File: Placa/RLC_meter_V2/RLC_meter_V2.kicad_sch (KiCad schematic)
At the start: 22 parts, among them J1 Batt1, J2 Batt2, J3 HC05, J4 Load_terminal, U1 LPC845, U2 X9Cxxx, U3 MC33202, U4 AMS1117-3.3

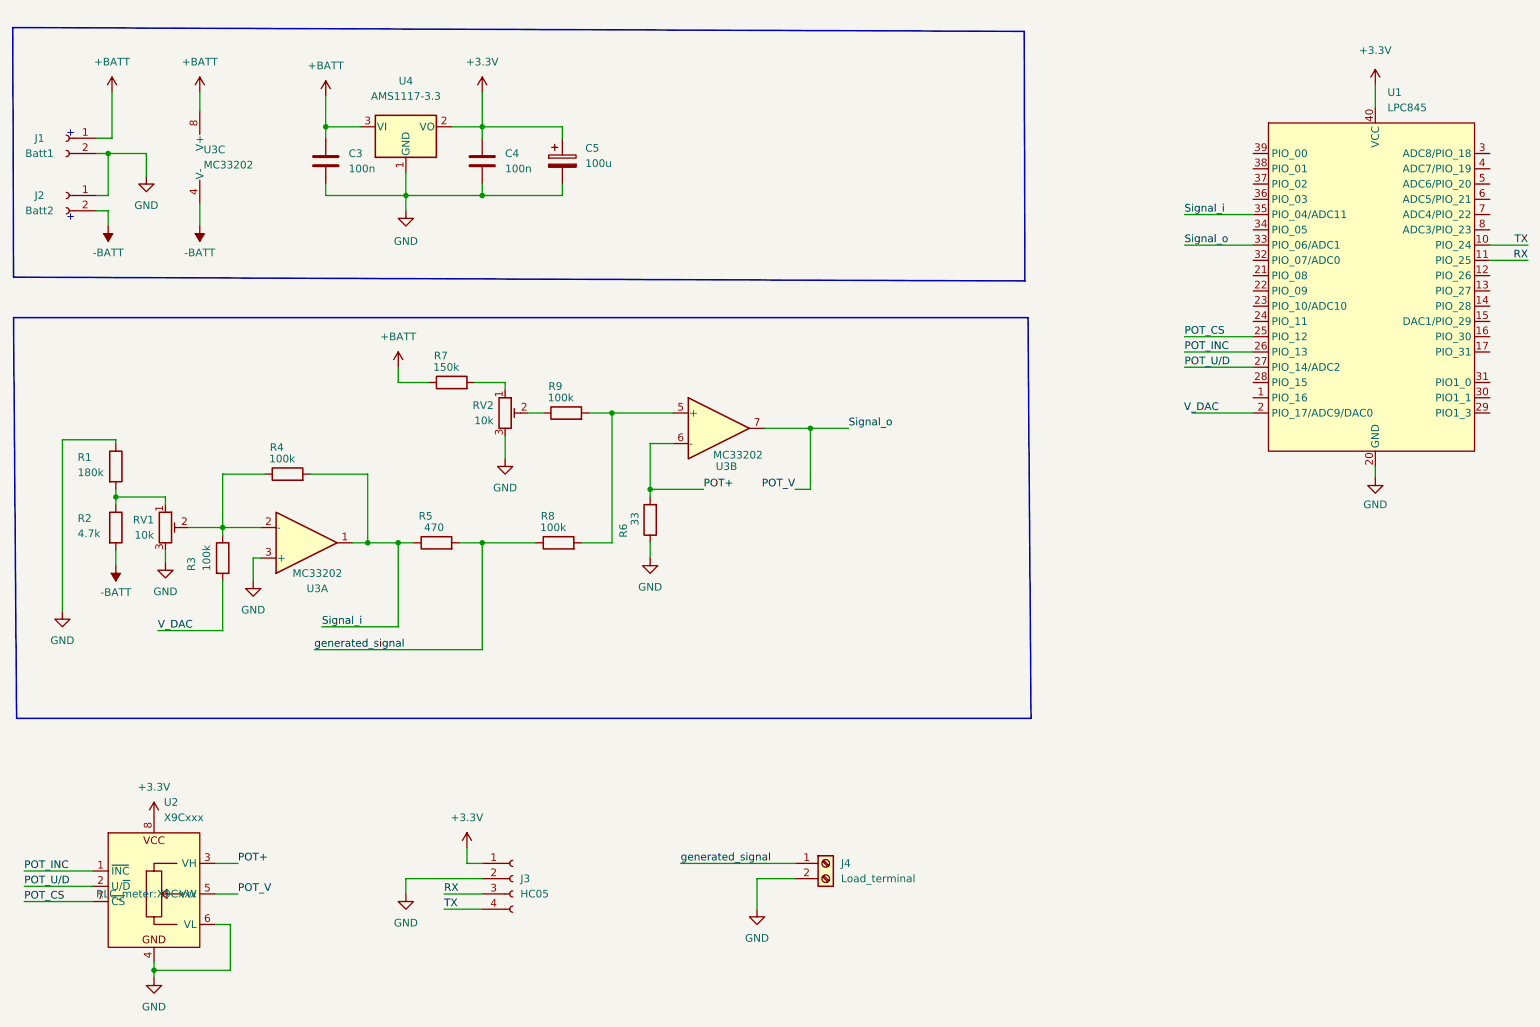
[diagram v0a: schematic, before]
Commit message: last commit
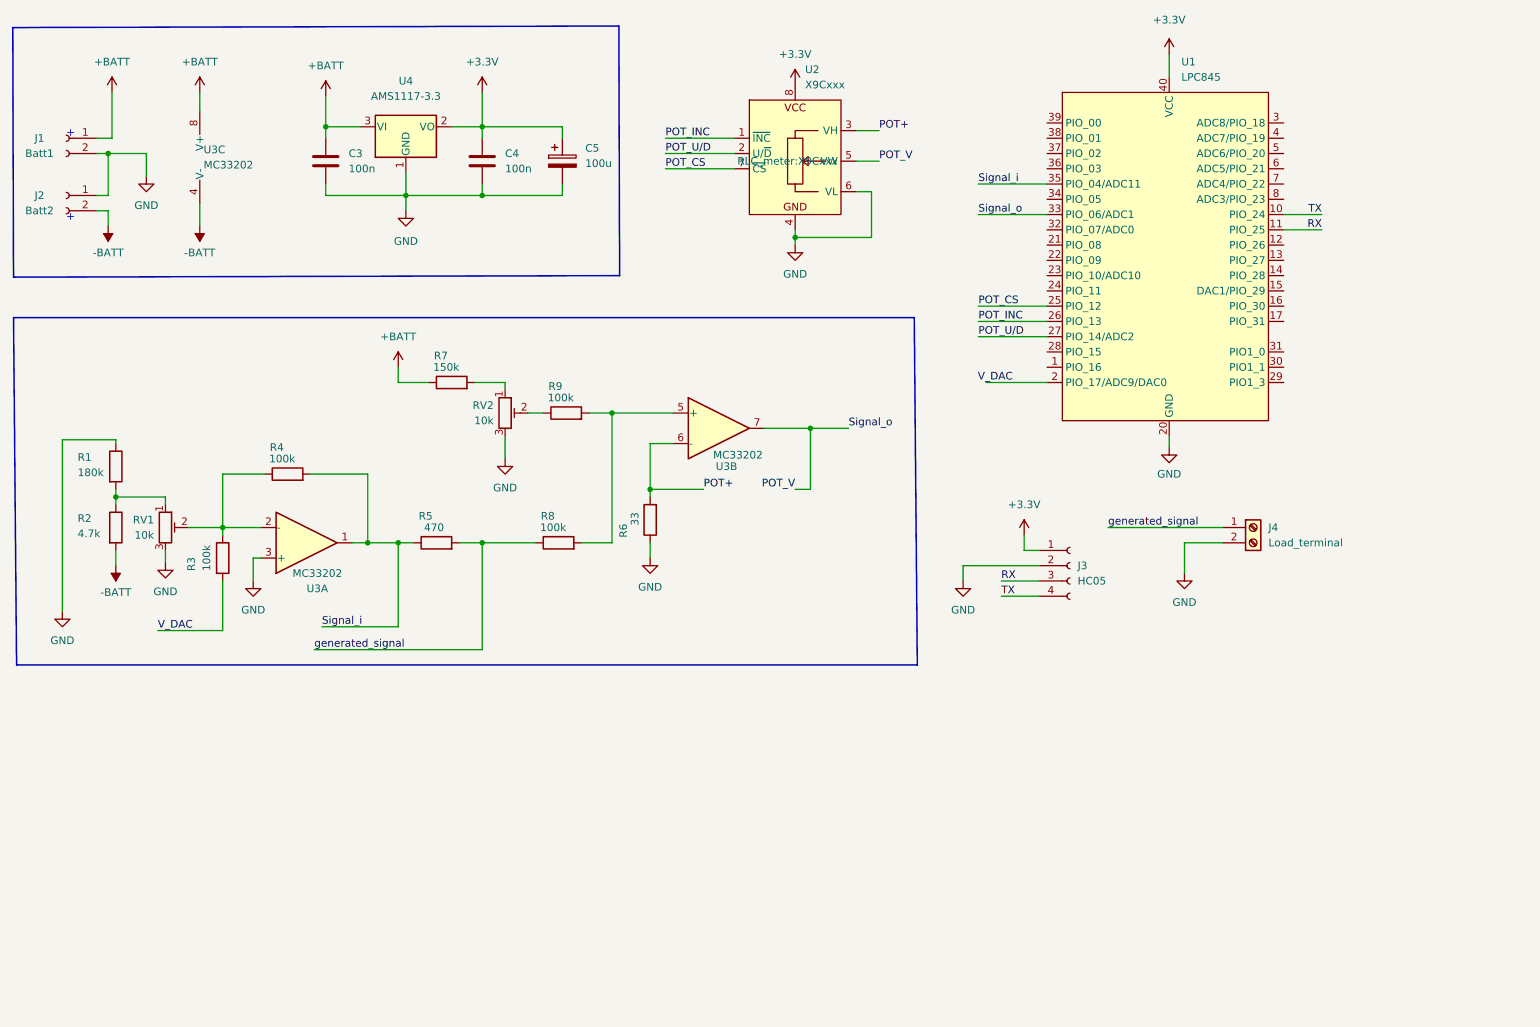
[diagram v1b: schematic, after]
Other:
- moved on the sheet: J3, J4, U1, U2
